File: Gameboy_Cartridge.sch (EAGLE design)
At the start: 10 parts, among them IC1 AT49F040J

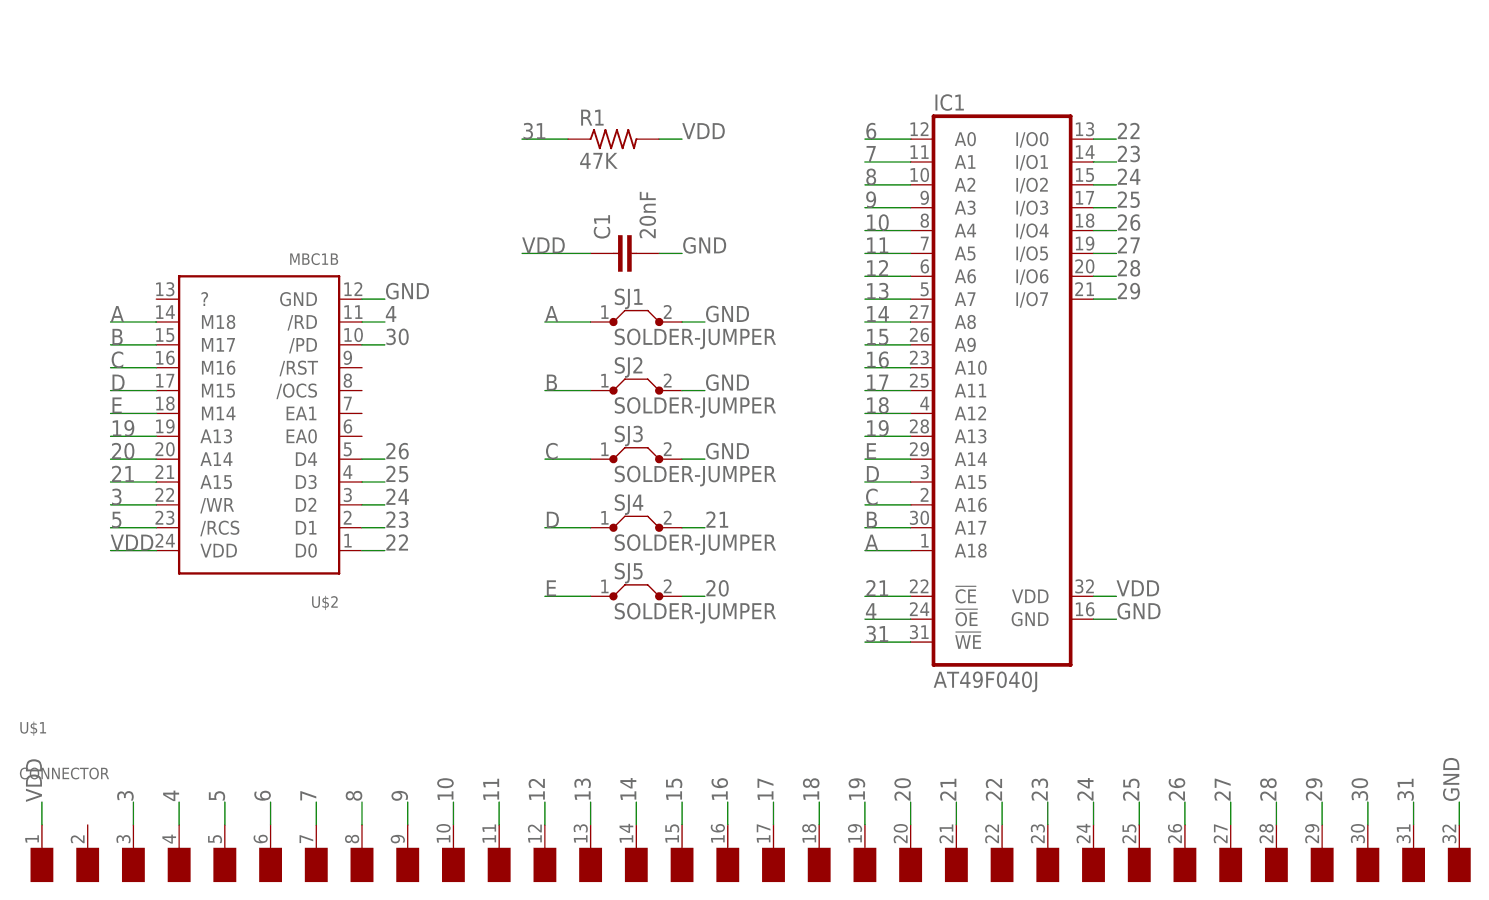
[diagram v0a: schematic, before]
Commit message: Changed a few details, hope I didn't screw it up...
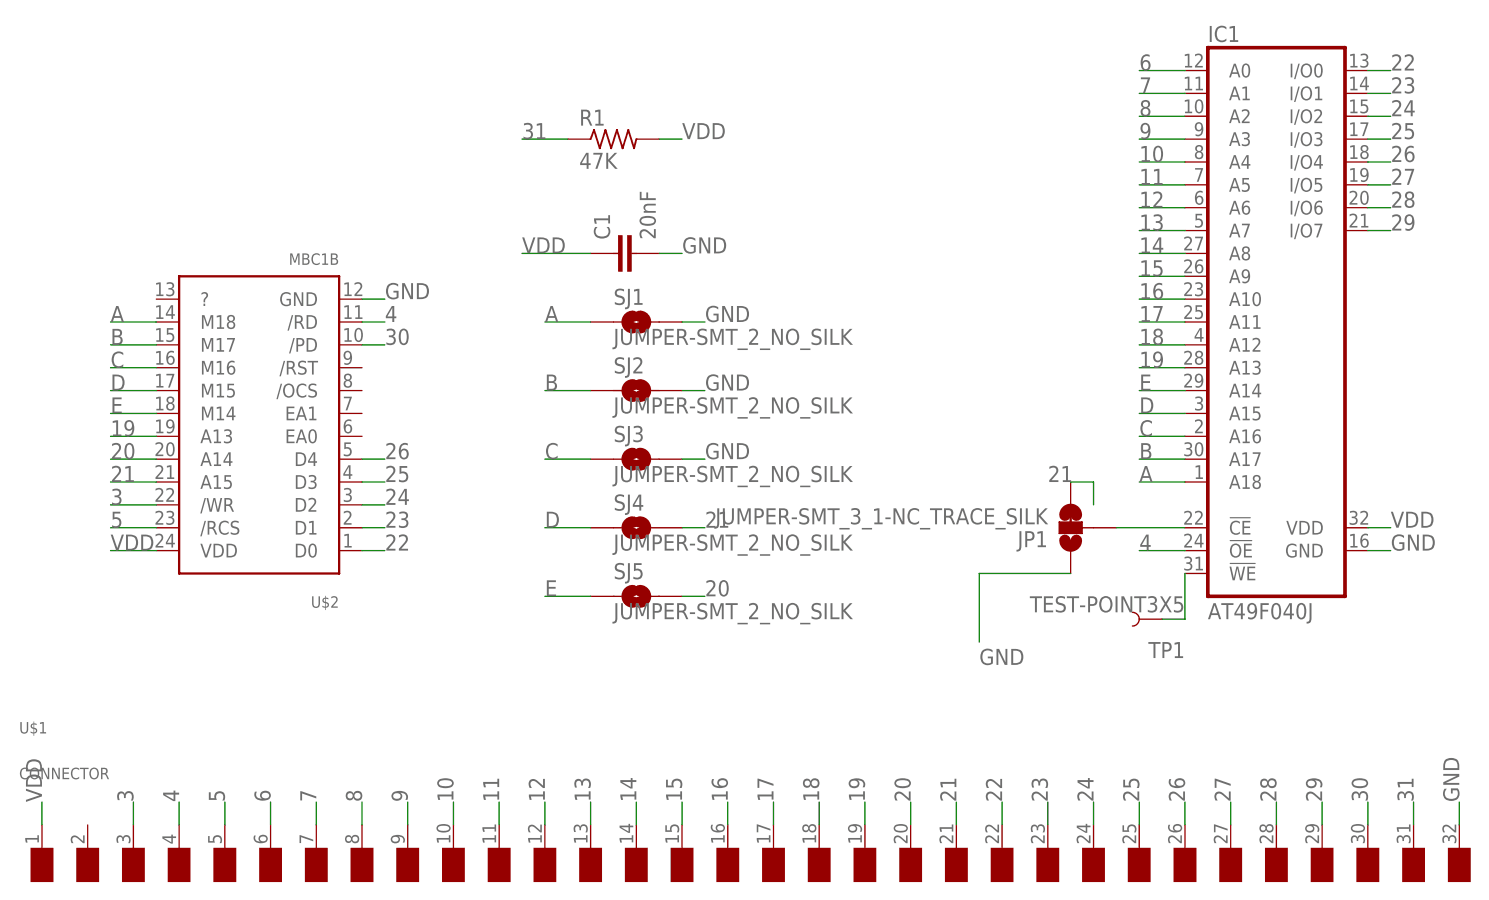
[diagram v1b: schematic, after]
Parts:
- added JP1: JUMPER-SMT_3_1-NC_TRACE_SILK, SparkFun-Jumpers:JUMPER-SMT_3_1-NC_TRACE_SILK
- added TP1: TEST-POINT3X5, SparkFun-Connectors:TEST-POINT3X5
- SJ1, SJ2, SJ3, SJ4, SJ5: value SOLDER-JUMPER -> JUMPER-SMT_2_NO_SILK; device gameboy:SOLDER-JUMPER -> SparkFun-Jumpers:JUMPER-SMT_2_NO_SILK
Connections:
- new net N$1: IC1.!WE, TP1.1
- new net N$2: IC1.!CE, JP1.2
- net 21: now also JP1.3; no longer IC1.!CE
- net 31: no longer IC1.!WE
- net GND: now also JP1.1
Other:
- moved on the sheet: IC1
